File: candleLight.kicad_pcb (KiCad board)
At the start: 2 copper layers, 37.7 x 20 mm, 44 parts, among them P501 USB_OTG, U201 STM32F072C8Tx, U301 MCP1754ST-3302E/MB, U401 TJA1051/3, X501 CON_SWD, X502 SUB-D9, Y201 8MHz

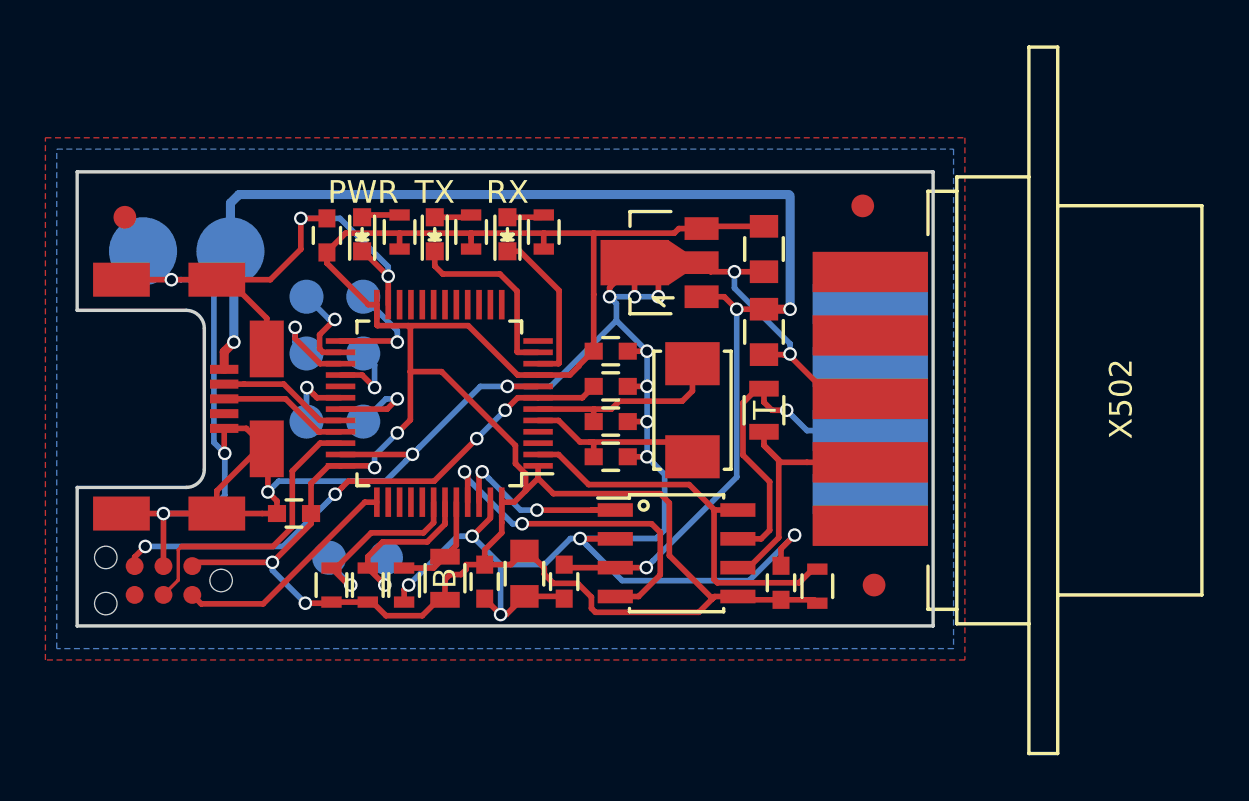
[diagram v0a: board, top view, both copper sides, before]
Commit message: fine tuning
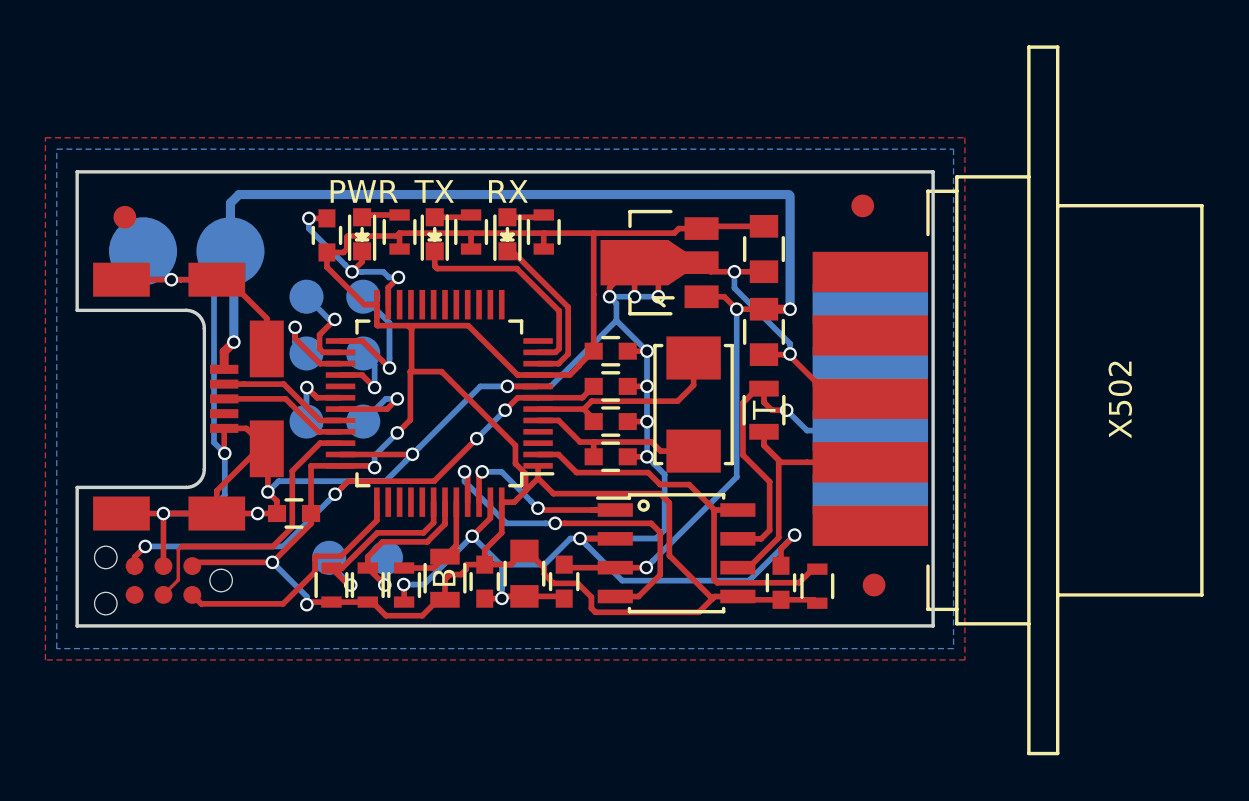
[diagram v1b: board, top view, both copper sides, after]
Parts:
- moved Y201 0.25 mm to (68.5, 85.2)
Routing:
- net GND: track 154.8 -> 147.5 mm, vias 22 -> 24
- net /LEDs/LED2: track 8.34 -> 9.60 mm
- net Net-(C201-Pad2): track 9.38 -> 8.17 mm
- net Net-(U201-Pad25): track 5.14 -> 6.27 mm
- net +3V3: track 115.2 -> 116.2 mm
- net /Connectors/SWCLK: track 10.1 -> 11.0 mm
